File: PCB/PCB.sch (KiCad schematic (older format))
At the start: 45 parts, among them J1 Conn_01x04_Female, J10 Conn_01x08_Female, J11 Conn_01x01_Female, J12 Conn_01x04_Female, J2 Conn_01x28_Female, J3 Conn_01x02_Female, J4 Conn_01x02_Female, J5 Conn_01x02_Female, J6 Conn_01x02_Female, J7 Conn_01x08_Female, J8 Conn_01x02_Female, J9 Conn_01x03_Female, Q1 PN2222A, Q2 IRF4905, U1 BA33BC0T, Y1 16MHz

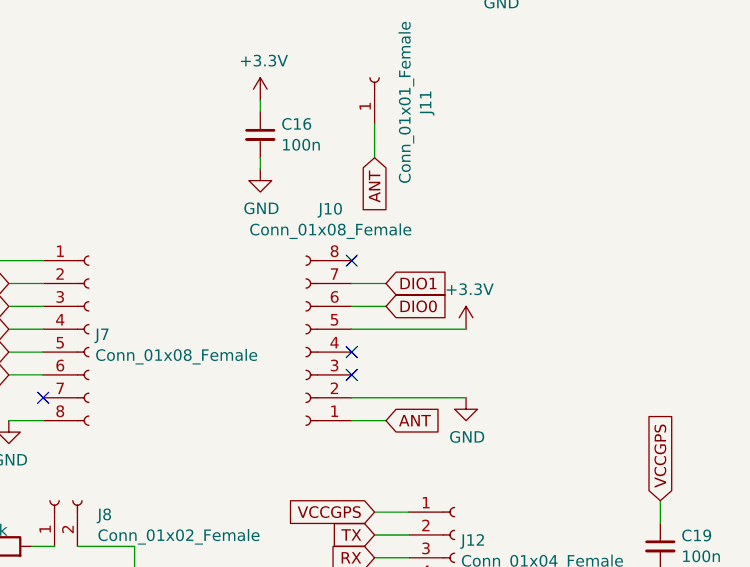
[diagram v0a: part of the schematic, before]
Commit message: Updated Schematic and PCB
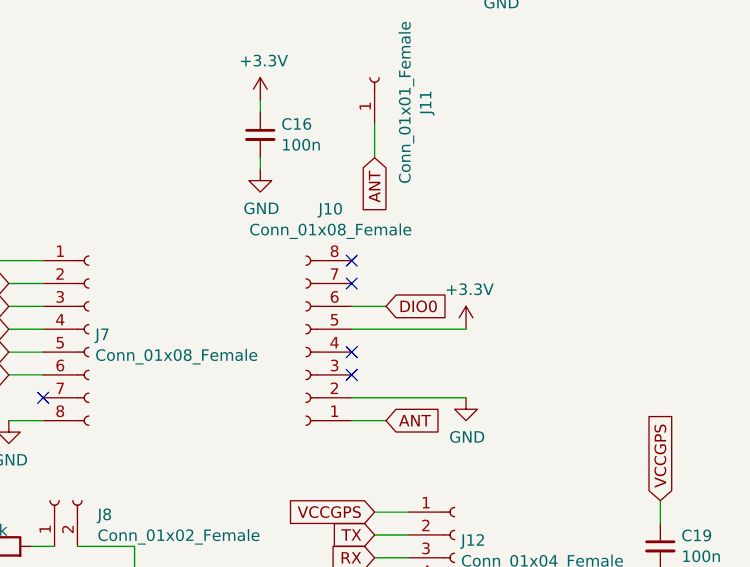
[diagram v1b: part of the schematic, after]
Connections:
- net DIO1: no longer names the net of J10.7 (Pin_7)
- no-connect marks 14 -> 15
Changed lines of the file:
@@
 NoConn ~ 8850 3400
 Wire Wire Line
-	9000 3100 8850 3100
-Wire Wire Line
 	9000 3200 8850 3200
 Wire Wire Line
 	9000 3700 8850 3700
-Text GLabel 9000 3100 2    50   Input ~ 0
-DIO1
 Text GLabel 9000 3200 2    50   Input ~ 0
 DIO0
@@
 Connection ~ 1650 1200
 Connection ~ 1650 1300
+NoConn ~ 8850 3100
 $EndSCHEMATC
